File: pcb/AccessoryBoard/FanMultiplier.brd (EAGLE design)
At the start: 38.1 x 38.1 mm, 26 parts, among them X1 M02PTH, X10 M02PTH, X11 M02PTH, X12 M02PTH, X3 M02PTH, X4 M02PTH, X5 M02PTH, X6 M02PTH, X7 M02PTH, X8 M02PTH, X9 M02PTH

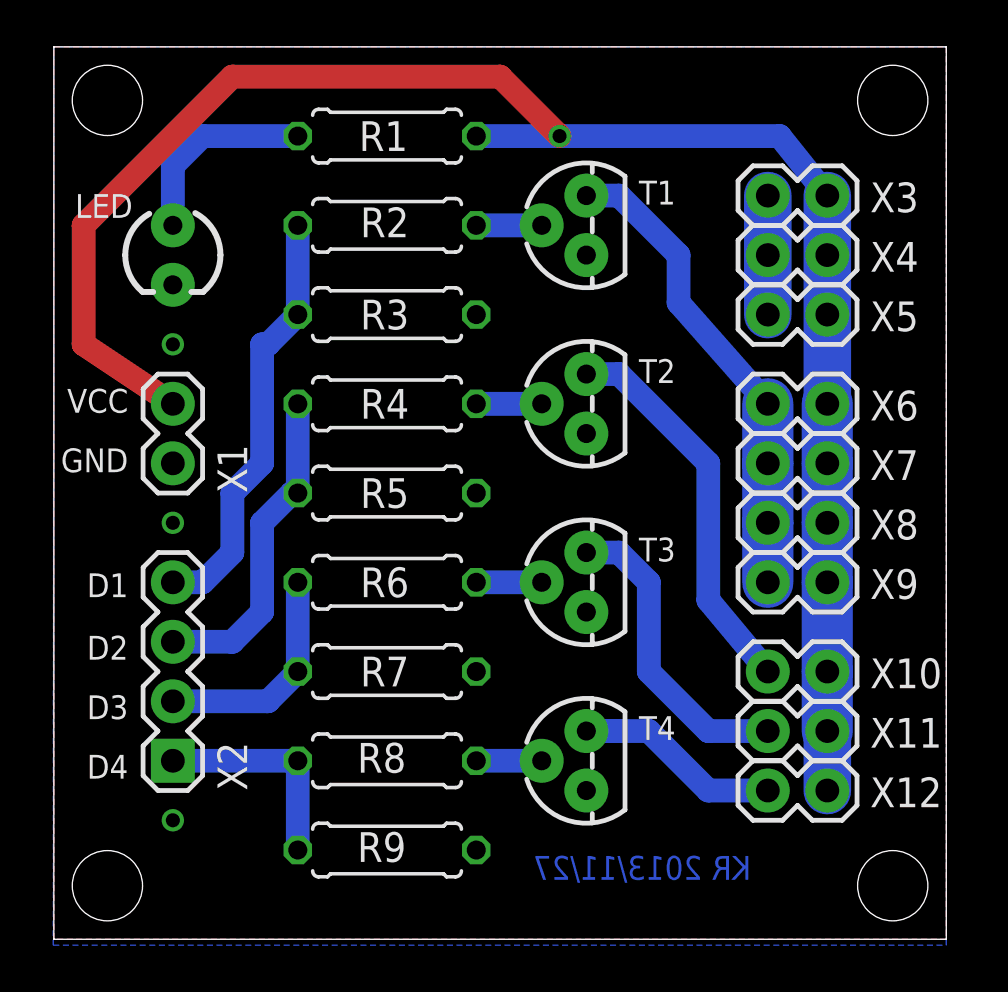
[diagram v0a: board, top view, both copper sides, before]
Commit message: brought headers together for easier soldering replaced logo with text other minor improvements
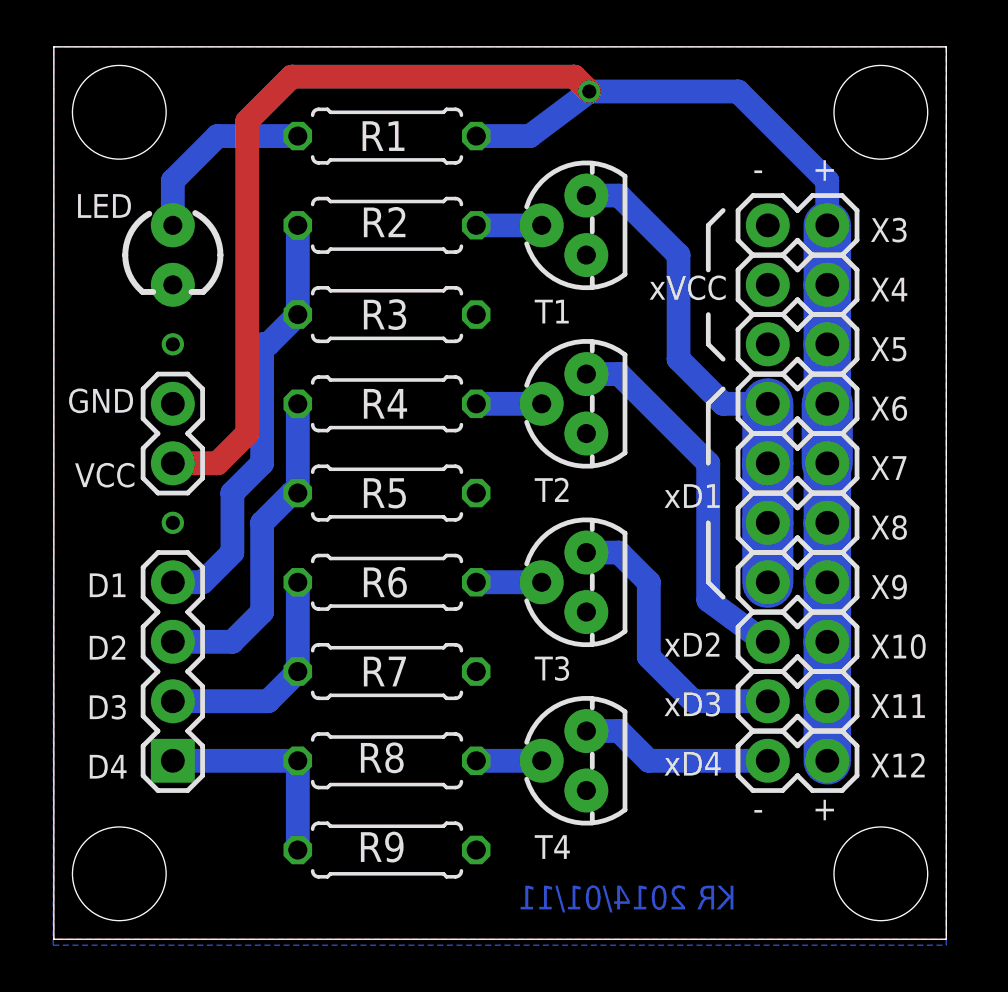
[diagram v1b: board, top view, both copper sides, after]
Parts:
- moved X1 2.54 mm to (5.08, 22.9), turned to 270 degrees
- moved X5 1.27 mm to (30.5, 25.4)
- moved X12 1.27 mm to (30.5, 7.62)
- moved X10 1.27 mm to (30.5, 12.7)
- moved X11 1.27 mm to (30.5, 10.2)
- moved X3 1.27 mm to (30.5, 30.5)
- moved X4 1.27 mm to (30.5, 27.9)
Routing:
- net GND: track 5.08 -> 0.00 mm, vias 0 -> 2
- net N$12: track 10.2 -> 8.27 mm
- net N$14: track 20.4 -> 21.7 mm
- net N$17: track 13.1 -> 12.2 mm
- net N$16: track 16.6 -> 15.8 mm
- net VCC: track 75.3 -> 74.7 mm
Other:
- board text added: "+"
- board text added: "-"
- board text added: "KR 2014/01/11"
- board text added: "Nova Labs Fan Board v4"
- board text added: "xD1"
- board text added: "xD2"
- board text added: "xD3"
- board text added: "xD4"
- board text added: "xVCC"
- board text removed: "KR 2013/11/27"
